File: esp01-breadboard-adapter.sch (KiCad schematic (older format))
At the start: 3 parts, among them P1 CONN_02X04, P2 CONN_01X10

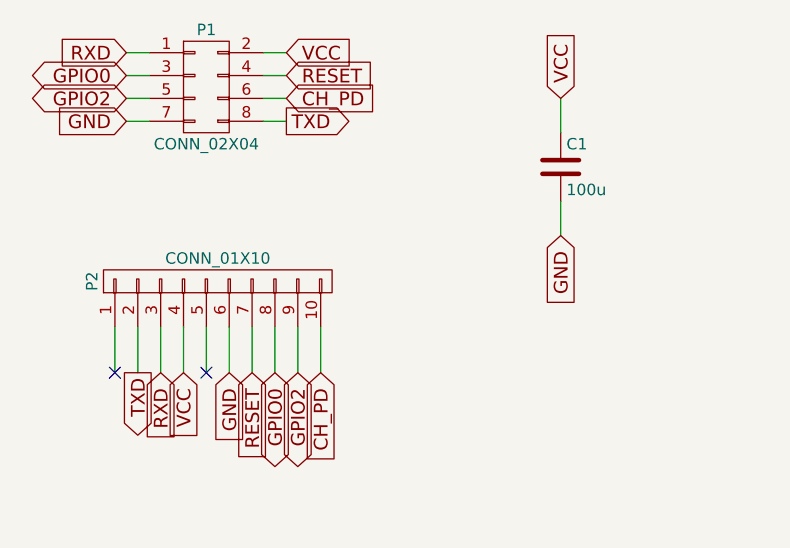
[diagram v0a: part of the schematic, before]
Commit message: added front silkscreen
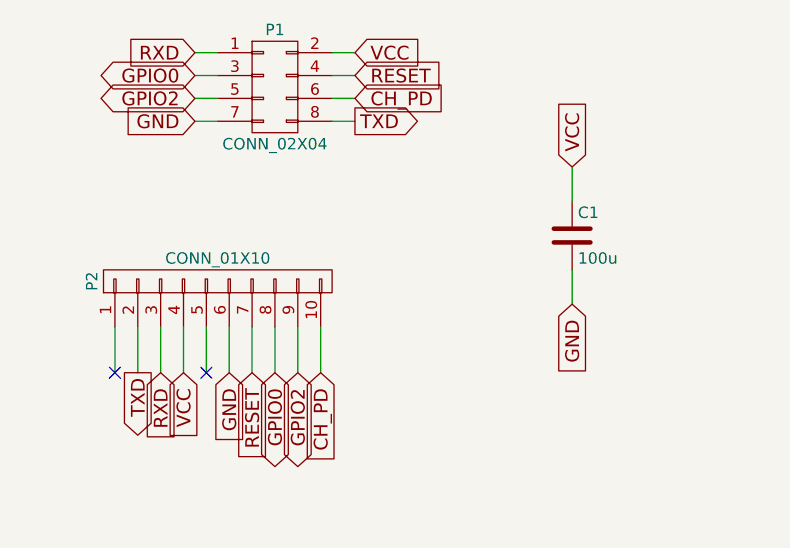
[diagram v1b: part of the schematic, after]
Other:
- moved on the sheet: C1, P1
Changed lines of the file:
@@
 L CONN_02X04 P1
 U 1 1 585E6580
-P 5650 3300
-F 0 "P1" H 5650 3550 50  0000 C CNN
-F 1 "CONN_02X04" H 5650 3050 50  0000 C CNN
-F 2 "Pin_Headers:Pin_Header_Straight_2x04" H 5650 2100 50  0001 C CNN
-F 3 "" H 5650 2100 50  0000 C CNN
-	1    5650 3300
+P 5950 3300
+F 0 "P1" H 5950 3550 50  0000 C CNN
+F 1 "CONN_02X04" H 5950 3050 50  0000 C CNN
+F 2 "Pin_Headers:Pin_Header_Straight_2x04" H 5950 2100 50  0001 C CNN
+F 3 "" H 5950 2100 50  0000 C CNN
+	1    5950 3300
 	1    0    0    -1
 $EndComp
 Wire Wire Line
-	5900 3150 6000 3150
+	6200 3150 6300 3150
 Wire Wire Line
-	5900 3250 6000 3250
+	6200 3250 6300 3250
 Wire Wire Line
-	5900 3350 6000 3350
+	6200 3350 6300 3350
 Wire Wire Line
-	5900 3450 6000 3450
+	6200 3450 6300 3450
 Wire Wire Line
-	5400 3450 5300 3450
+	5700 3450 5600 3450
 Wire Wire Line
-	5400 3350 5300 3350
+	5700 3350 5600 3350
 Wire Wire Line
-	5400 3250 5300 3250
+	5700 3250 5600 3250
 Wire Wire Line
-	5400 3150 5300 3150
-Text GLabel 6000 3150 2    60   Input ~ 0
+	5700 3150 5600 3150
+Text GLabel 6300 3150 2    60   Input ~ 0
 VCC
-Text GLabel 6000 3250 2    60   Input ~ 0
+Text GLabel 6300 3250 2    60   Input ~ 0
 RESET
-Text GLabel 6000 3350 2    60   Input ~ 0
+Text GLabel 6300 3350 2    60   Input ~ 0
 CH_PD
-Text GLabel 6000 3450 2    60   Output ~ 0
+Text GLabel 6300 3450 2    60   Output ~ 0
 TXD
-Text GLabel 5300 3150 0    60   Input ~ 0
+Text GLabel 5600 3150 0    60   Input ~ 0
 RXD
-Text GLabel 5300 3250 0    60   BiDi ~ 0
+Text GLabel 5600 3250 0    60   BiDi ~ 0
 GPIO0
-Text GLabel 5300 3350 0    60   BiDi ~ 0
+Text GLabel 5600 3350 0    60   BiDi ~ 0
 GPIO2
-Text GLabel 5300 3450 0    60   Input ~ 0
+Text GLabel 5600 3450 0    60   Input ~ 0
 GND
 $Comp
 L C C1
 U 1 1 585F8F92
-P 7200 3650
-F 0 "C1" H 7225 3750 50  0000 L CNN
-F 1 "100u" H 7225 3550 50  0000 L CNN
-F 2 "Capacitors_SMD:C_1206" H 7238 3500 50  0001 C CNN
-F 3 "" H 7200 3650 50  0000 C CNN
-	1    7200 3650
+P 7250 3950
+F 0 "C1" H 7275 4050 50  0000 L CNN
+F 1 "100u" H 7275 3850 50  0000 L CNN
+F 2 "Capacitors_SMD:C_1206" H 7288 3800 50  0001 C CNN
+F 3 "" H 7250 3950 50  0000 C CNN
+	1    7250 3950
 	1    0    0    -1
 $EndComp
 Wire Wire Line
-	7200 3500 7200 3350
+	7250 3800 7250 3650
 Wire Wire Line
-	7200 3800 7200 3950
-Text GLabel 7200 3350 1    60   Input ~ 0
+	7250 4100 7250 4250
+Text GLabel 7250 3650 1    60   Input ~ 0
 VCC
-Text GLabel 7200 3950 3    60   Input ~ 0
+Text GLabel 7250 4250 3    60   Input ~ 0
 GND
 Text Notes 7350 7500 0    60   ~ 0
